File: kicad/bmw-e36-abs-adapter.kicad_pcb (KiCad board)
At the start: 0 parts

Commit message: Initial placement on PCB
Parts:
- added C1: 10u, Capacitor_SMD:C_1206_3216Metric, F.Cu at (241.0, 130.0)
- added C10: 10u, Capacitor_SMD:C_1206_3216Metric, F.Cu at (216.0, 174.0)
- added C11: 0.1u, Capacitor_SMD:C_0603_1608Metric, F.Cu at (221.0, 166.3)
- added C12: 12p, Capacitor_SMD:C_0603_1608Metric, F.Cu at (217.0, 179.0)
- added C13: 0.1u, Capacitor_SMD:C_0603_1608Metric, F.Cu at (215.0, 176.0)
- added C14: 12p, Capacitor_SMD:C_0603_1608Metric, F.Cu at (223.0, 179.0)
- added C15: 1u, Capacitor_SMD:C_0603_1608Metric, F.Cu at (203.0, 173.0)
- added C16: 0.01u, Capacitor_SMD:C_0603_1608Metric, F.Cu at (203.0, 175.0)
- added C17: 0.1u, Capacitor_SMD:C_0603_1608Metric, F.Cu at (179.0, 111.0)
- added C18: 0.1u, Capacitor_SMD:C_0603_1608Metric, F.Cu at (224.0, 117.0)
- added C19: 0.1u, Capacitor_SMD:C_0603_1608Metric, F.Cu at (219.0, 117.0)
- added C2: 1u, Capacitor_SMD:C_0603_1608Metric, F.Cu at (242.0, 122.0)
- added C20: 0.1u, Capacitor_SMD:C_0603_1608Metric, F.Cu at (186.0, 122.0)
- added C3: 10u, Capacitor_SMD:C_1206_3216Metric, F.Cu at (253.0, 142.0)
- added C4: 47u, Capacitor_SMD:CP_Elec_8x6.5, F.Cu at (241.1, 109.0)
- added C5: 22u, Capacitor_SMD:C_1206_3216Metric, F.Cu at (248.0, 126.0)
- added C6: 0.1u, Capacitor_SMD:C_0603_1608Metric, F.Cu at (238.8, 115.0)
- added C7: 10u, Capacitor_SMD:C_1206_3216Metric, F.Cu at (241.0, 142.0)
- added C8: 10u, Capacitor_SMD:C_1206_3216Metric, F.Cu at (211.0, 184.0)
- added C9: 0.1u, Capacitor_SMD:C_0603_1608Metric, F.Cu at (213.0, 183.0)
- added D1: NRVBA340NT3G, Diode_SMD:D_SMA, F.Cu at (238.0, 97.0)
- added D2: VTVS40ASMF-HM3-08, Diode_SMD:D_SMF, F.Cu at (239.4, 103.0)
- added D3: RED, LED_SMD:LED_0603_1608Metric, F.Cu at (238.0, 142.0)
- added D4: GREEN, LED_SMD:LED_0603_1608Metric, F.Cu at (213.0, 166.0)
- added D5: SZNUP2105LT3G, Package_TO_SOT_SMD:SOT-23, F.Cu at (185.0, 107.0)
- added D6: BZX38450-C3V3-Q, Diode_SMD:D_SOD-323, F.Cu at (224.0, 125.0)
- added D7: BZX38450-C3V3-Q, Diode_SMD:D_SOD-323, F.Cu at (219.0, 125.0)
- added D8: VTVS40ASMF-HM3-08, Diode_SMD:D_SMF, F.Cu at (202.0, 123.0)
- added D9: VTVS40ASMF-HM3-08, Diode_SMD:D_SMF, F.Cu at (209.0, 123.0)
- added F1: 500mA, Fuse:Fuse_1206_3216Metric, F.Cu at (227.0, 108.0)
- added F2: 20mA, Fuse:Fuse_0603_1608Metric, F.Cu at (186.0, 120.0)
- added H1: MountingHole, MountingHole:MountingHole_3.2mm_M3, F.Cu at (165.0, 95.0)
- added H2: MountingHole, MountingHole:MountingHole_3.2mm_M3, F.Cu at (255.0, 95.0)
- added H3: MountingHole, MountingHole:MountingHole_3.2mm_M3, F.Cu at (165.0, 185.0)
- added H4: MountingHole, MountingHole:MountingHole_3.2mm_M3, F.Cu at (255.0, 185.0)
- added J1: TE_9-6437287-8, bmw-e36-abs-adapter:TE_9-6437287-8, F.Cu at (210.0, 93.0)
- added J2: SWD, Connector:Tag-Connect_TC2030-IDC-NL_2x03_P1.27mm_Vertical, F.Cu at (204.0, 164.0)
- added JP1: RST, Jumper:SolderJumper-2_P1.3mm_Open_RoundedPad1.0x1.5mm, F.Cu at (218.0, 166.3)
- added JP2: BOOT, Jumper:SolderJumper-2_P1.3mm_Open_RoundedPad1.0x1.5mm, F.Cu at (218.0, 184.0)
- added JP3: TERM, Connector_PinHeader_2.54mm:PinHeader_1x02_P2.54mm_Vertical, F.Cu at (190.0, 107.0)
- added NT1: NetTie_2, NetTie:NetTie-2_SMD_Pad0.5mm, F.Cu at (225.0, 108.0)
- added Q1: BSS138, Package_TO_SOT_SMD:SOT-323_SC-70, F.Cu at (200.0, 140.0)
- added Q2: BSS138, Package_TO_SOT_SMD:SOT-323_SC-70, F.Cu at (203.0, 142.0)
- added Q3: BSS138, Package_TO_SOT_SMD:SOT-323_SC-70, F.Cu at (197.0, 140.0)
- added Q4: BSS138, Package_TO_SOT_SMD:SOT-323_SC-70, F.Cu at (203.0, 133.0)
- added Q5: BSS138, Package_TO_SOT_SMD:SOT-323_SC-70, F.Cu at (200.0, 131.0)
- added Q6: BSS138, Package_TO_SOT_SMD:SOT-323_SC-70, F.Cu at (208.0, 142.0)
- added Q7: BSS138, Package_TO_SOT_SMD:SOT-323_SC-70, F.Cu at (208.0, 133.0)
- added R1: 1k, Resistor_SMD:R_0603_1608Metric, F.Cu at (238.0, 146.0)
- added R10: 10k, Resistor_SMD:R_0603_1608Metric, F.Cu at (224.0, 123.0)
- added R11: 10k, Resistor_SMD:R_0603_1608Metric, F.Cu at (219.0, 123.0)
- added R12: 130, Resistor_SMD:R_0603_1608Metric, F.Cu at (175.0, 125.0)
- added R13: 130, Resistor_SMD:R_0603_1608Metric, F.Cu at (175.0, 130.0)
- added R14: 130, Resistor_SMD:R_0603_1608Metric, F.Cu at (175.0, 135.0)
- added R15: 130, Resistor_SMD:R_0603_1608Metric, F.Cu at (175.0, 140.0)
- added R16: 130, Resistor_SMD:R_0603_1608Metric, F.Cu at (175.0, 145.0)
- added R17: 130, Resistor_SMD:R_0603_1608Metric, F.Cu at (175.0, 150.0)
- added R18: 249, Resistor_SMD:R_0603_1608Metric, F.Cu at (185.0, 125.0)
- added R19: 187, Resistor_SMD:R_0603_1608Metric, F.Cu at (185.0, 130.0)
- added R2: 22, Resistor_SMD:R_0603_1608Metric, F.Cu at (206.0, 168.0)
- added R20: 127, Resistor_SMD:R_0603_1608Metric, F.Cu at (185.0, 135.0)
- added R21: 127, Resistor_SMD:R_0603_1608Metric, F.Cu at (185.0, 140.0)
- added R22: 127, Resistor_SMD:R_0603_1608Metric, F.Cu at (185.0, 145.0)
- added R23: 215, Resistor_SMD:R_0603_1608Metric, F.Cu at (185.0, 150.0)
- added R24: 10k, Resistor_SMD:R_0603_1608Metric, F.Cu at (203.0, 145.0)
- added R25: 10k, Resistor_SMD:R_0603_1608Metric, F.Cu at (199.0, 143.0)
- added R26: 10k, Resistor_SMD:R_0603_1608Metric, F.Cu at (203.0, 139.0)
- added R27: 10k, Resistor_SMD:R_0603_1608Metric, F.Cu at (199.0, 134.0)
- added R28: 10k, Resistor_SMD:R_0603_1608Metric, F.Cu at (203.0, 130.0)
- added R29: 10k, Resistor_SMD:R_0603_1608Metric, F.Cu at (208.0, 145.0)
- added R3: 22, Resistor_SMD:R_0603_1608Metric, F.Cu at (204.0, 168.0)
- added R30: 10k, Resistor_SMD:R_0603_1608Metric, F.Cu at (208.0, 139.0)
- added R31: 10k, Resistor_SMD:R_0603_1608Metric, F.Cu at (208.0, 130.0)
- added R4: 1k, Resistor_SMD:R_0603_1608Metric, F.Cu at (211.0, 166.0)
- added R5: 120, Resistor_SMD:R_0603_1608Metric, F.Cu at (190.0, 103.0)
- added R6: 0, Resistor_SMD:R_0603_1608Metric, F.Cu at (225.0, 114.0)
- added R7: 0, Resistor_SMD:R_0603_1608Metric, F.Cu at (220.0, 114.0)
- added R8: 5.6k, Resistor_SMD:R_0603_1608Metric, F.Cu at (225.0, 120.0)
- added R9: 5.6k, Resistor_SMD:R_0603_1608Metric, F.Cu at (220.0, 120.0)
- added TP1: TestPoint, TestPoint:TestPoint_Keystone_5000-5004_Miniature, F.Cu at (254.0, 105.0)
- added TP10: TestPoint, TestPoint:TestPoint_Pad_D1.5mm, F.Cu at (199.0, 137.0)
- added TP11: TestPoint, TestPoint:TestPoint_Pad_D1.5mm, F.Cu at (203.0, 136.0)
- added TP12: TestPoint, TestPoint:TestPoint_Pad_D1.5mm, F.Cu at (203.0, 127.0)
- added TP13: TestPoint, TestPoint:TestPoint_Pad_D1.5mm, F.Cu at (208.0, 148.0)
- added TP14: TestPoint, TestPoint:TestPoint_Pad_D1.5mm, F.Cu at (208.0, 136.0)
- added TP15: TestPoint, TestPoint:TestPoint_Pad_D1.5mm, F.Cu at (208.0, 127.0)
- added TP2: TestPoint, TestPoint:TestPoint_Pad_D1.5mm, F.Cu at (247.0, 130.0)
- added TP3: TestPoint, TestPoint:TestPoint_Pad_D1.5mm, F.Cu at (239.0, 138.0)
- added TP4: TestPoint, TestPoint:TestPoint_Pad_D1.5mm, F.Cu at (173.0, 109.0)
- added TP5: TestPoint, TestPoint:TestPoint_Pad_D1.5mm, F.Cu at (173.0, 105.0)
- added TP6: TestPoint, TestPoint:TestPoint_Pad_D1.5mm, F.Cu at (225.0, 128.0)
- added TP7: TestPoint, TestPoint:TestPoint_Pad_D1.5mm, F.Cu at (220.0, 128.0)
- added TP8: TestPoint, TestPoint:TestPoint_Pad_D1.5mm, F.Cu at (199.0, 146.0)
- added TP9: TestPoint, TestPoint:TestPoint_Pad_D1.5mm, F.Cu at (203.0, 148.0)
- added U1: TPSM33610S5, bmw-e36-abs-adapter:Texas_RDN0011B_QFN-FCMOD-11-3.5x4.5mm-P0.5mm_2EP, F.Cu at (243.0, 126.0)
- added U10: VOMA617A-8X001T, bmw-e36-abs-adapter:SOP-4_4.4x4.6mm_P2.54mm, F.Cu at (180.0, 150.0)
- added U2: TLE42744DV33ATMA1, Package_TO_SOT_SMD:TO-252-2, F.Cu at (247.0, 145.0)
- added U3: STM32F042K6Ux, Package_DFN_QFN:QFN-32-1EP_5x5mm_P0.5mm_EP3.45x3.45mm, F.Cu at (209.0, 177.0)
- added U4: TCAN3404DRQ1, Package_SO:JEITA_SOIC-8_3.9x4.9mm_P1.27mm, F.Cu at (179.0, 107.0)
- added U5: VOMA617A-8X001T, bmw-e36-abs-adapter:SOP-4_4.4x4.6mm_P2.54mm, F.Cu at (180.0, 125.0)
- added U6: VOMA617A-8X001T, bmw-e36-abs-adapter:SOP-4_4.4x4.6mm_P2.54mm, F.Cu at (180.0, 130.0)
- added U7: VOMA617A-8X001T, bmw-e36-abs-adapter:SOP-4_4.4x4.6mm_P2.54mm, F.Cu at (180.0, 135.0)
- added U8: VOMA617A-8X001T, bmw-e36-abs-adapter:SOP-4_4.4x4.6mm_P2.54mm, F.Cu at (180.0, 140.0)
- added U9: VOMA617A-8X001T, bmw-e36-abs-adapter:SOP-4_4.4x4.6mm_P2.54mm, F.Cu at (180.0, 145.0)
- added Y1: ECS-160-10-36Q-AES-TR, Crystal:Crystal_SMD_2520-4Pin_2.5x2.0mm, F.Cu at (220.0, 179.0)
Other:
- board outline added: 100 x 100 mm
- copper layers 0 -> 2

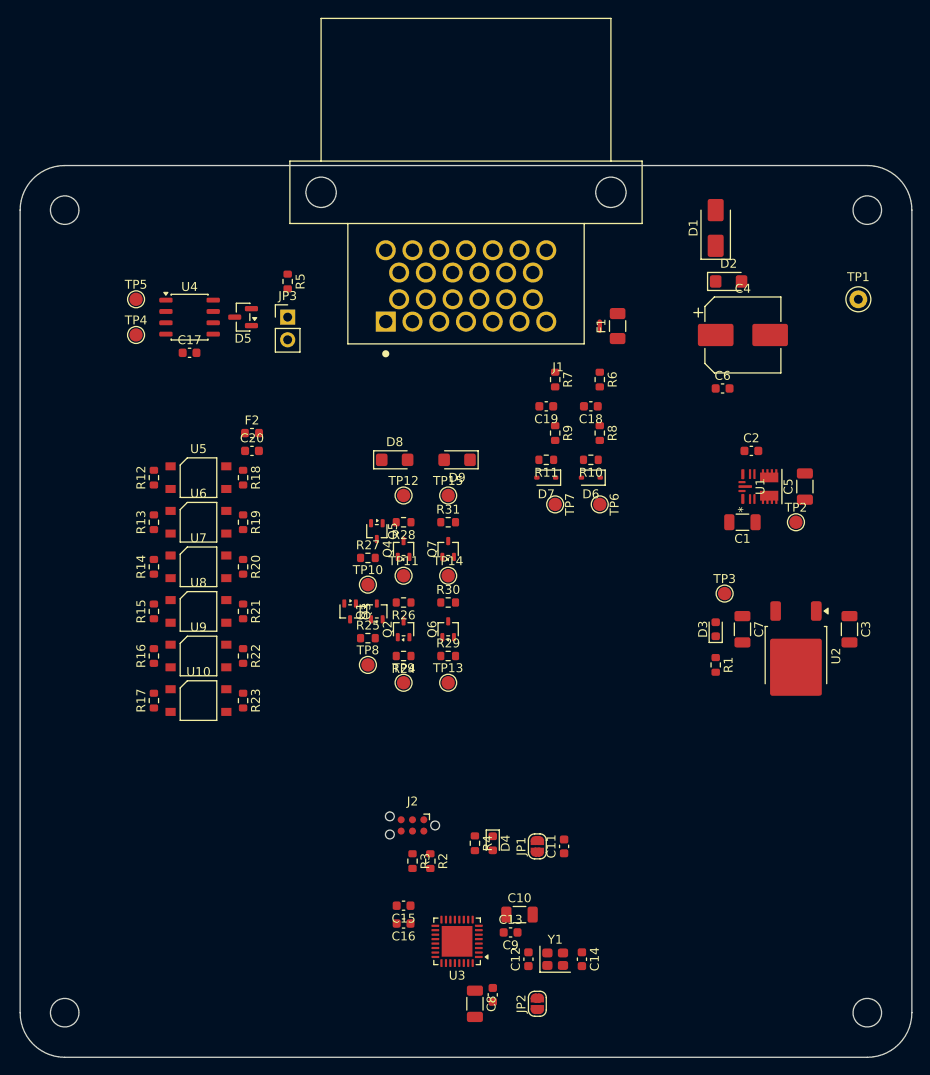
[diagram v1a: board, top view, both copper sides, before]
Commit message: PCB Design WIP
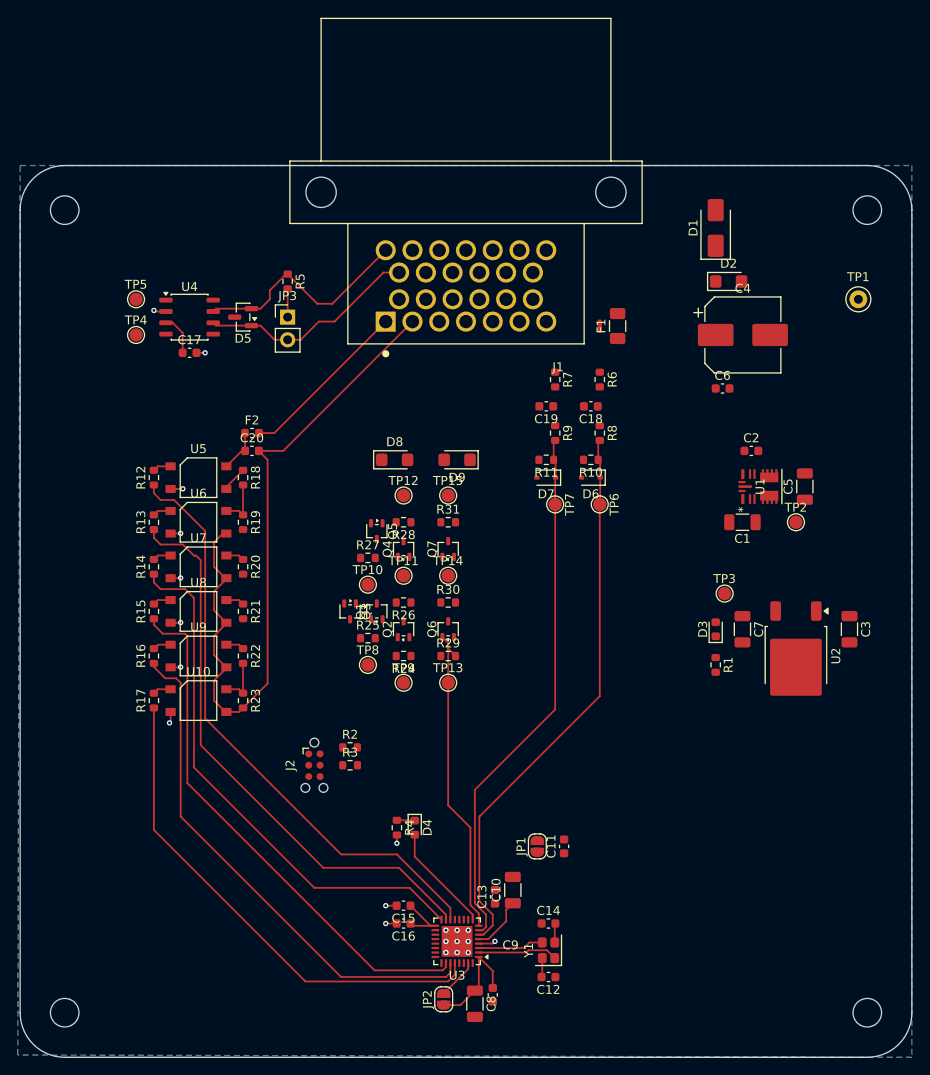
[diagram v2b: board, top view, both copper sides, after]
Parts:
- moved R2 15.6 mm to (197.0, 155.2), turned to 0 degrees
- moved J2 12.9 mm to (193.0, 157.2), turned to -90 degrees
- moved R3 12.8 mm to (197.0, 157.2), turned to 0 degrees
- moved JP2 10.5 mm to (207.5, 183.5)
- moved D4 8.92 mm to (204.2, 164.2)
- moved R4 8.92 mm to (202.2, 164.2)
- moved C14 5.48 mm to (219.2, 175.0), turned to 0 degrees
- moved C13 4.37 mm to (213.2, 172.0), turned to 90 degrees
- moved C12 3.01 mm to (219.2, 181.0), turned to 180 degrees
- moved C10 2.85 mm to (215.2, 171.2), turned to 90 degrees
- moved Y1 1.25 mm to (219.2, 178.0), turned to 90 degrees
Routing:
- net /PEDAL_T2: track 0.00 -> 80.6 mm
- net /PEDAL_EN: track 0.00 -> 67.1 mm
- net /PEDAL_L0: track 0.00 -> 63.9 mm
- net /PRES_1_3V3: track 0.00 -> 62.8 mm
- net /PEDAL_L1: track 0.00 -> 60.0 mm
- net /PRES_2_3V3: track 0.00 -> 60.0 mm
- net /PEDAL_L2: track 0.00 -> 59.7 mm
- net /PEDAL_L3: track 0.00 -> 58.1 mm
- net /PEDAL_L4: track 0.00 -> 56.1 mm
- net /L_LINE_TX: track 0.00 -> 35.2 mm
- net +3.3V: track 0.00 -> 29.7 mm
- net /CAN_H: track 0.00 -> 25.5 mm
- net /CAN_L: track 0.00 -> 24.8 mm
- net /PEDAL_T1: track 0.00 -> 19.4 mm
- net GND: track 0.00 -> 17.3 mm, vias 0 -> 20
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- added copper zone on B.Cu, net GND
